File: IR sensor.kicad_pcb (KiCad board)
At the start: 2 copper layers, 33.5 x 16.8 mm, 23 parts, among them P1 BNC, P2 BNC, P3 BNC, P4 CONN_01X02, Q1 SOT-23-3 NPN, U1 TLV2770IDGKR, U2 LM311MX/NOPB

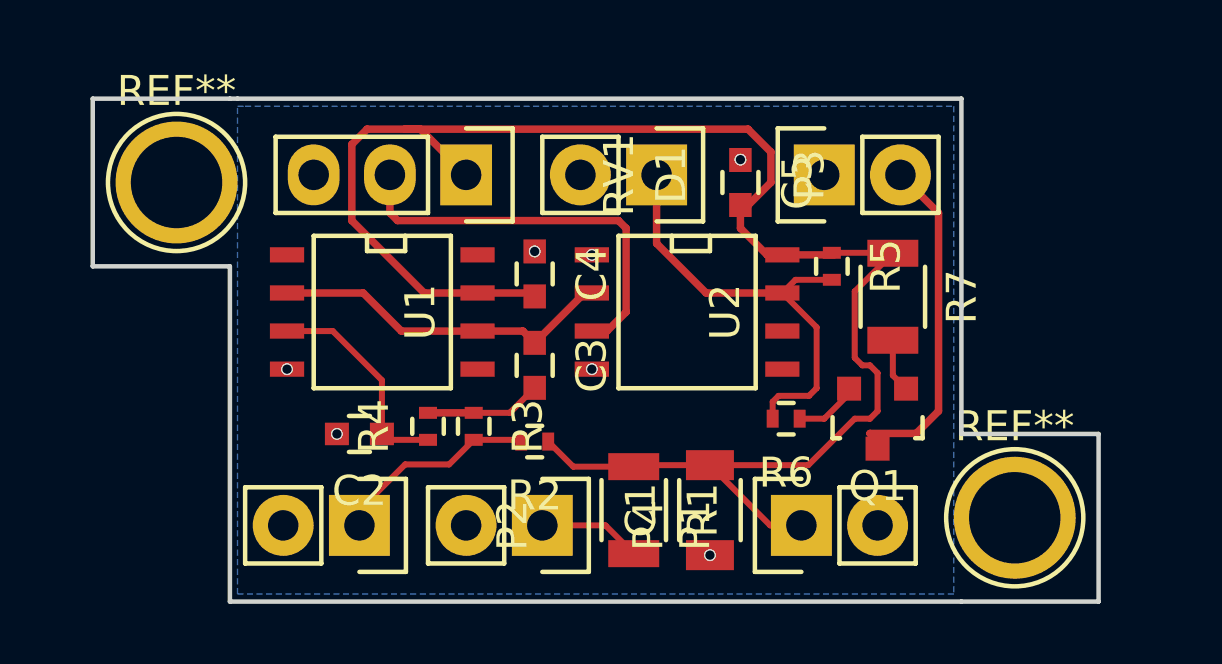
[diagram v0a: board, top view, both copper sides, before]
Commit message: ENH: Updates to IR sensors
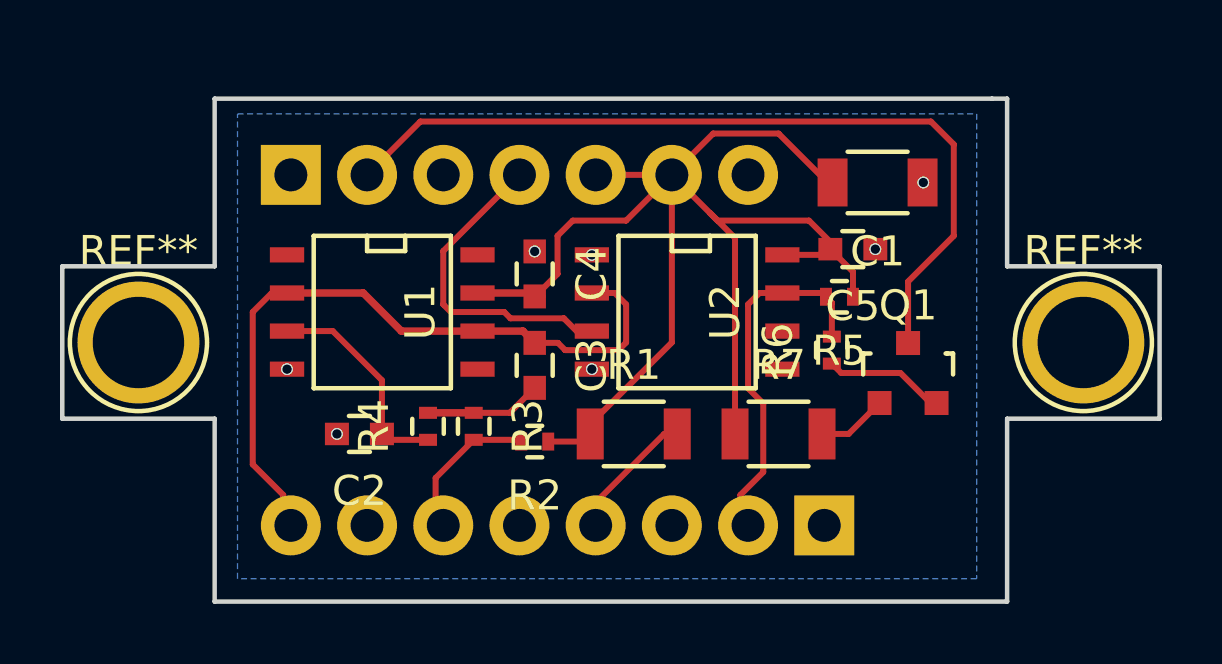
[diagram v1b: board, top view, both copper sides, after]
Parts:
- removed D1: LED, Pin_Headers:Pin_Header_Straight_1x02
- removed P3: BNC, Pin_Headers:Pin_Header_Straight_1x02
- removed P4: CONN_01X02, Pin_Headers:Pin_Header_Straight_1x02
- removed the REF** at (142.0, 67.3)
- removed the REF** at (169.9, 78.5)
- removed RV1: POT, Pin_Headers:Pin_Header_Straight_1x03
- added REF**: 1pin, Connect:1pin, F.Cu at (172.2, 72.6)
- added REF**: 1pin, Connect:1pin, F.Cu at (140.7, 72.6)
- P1: value BNC -> CONN_01X08; footprint Pin_Headers:Pin_Header_Straight_1x02 -> Terminal_Blocks:TerminalBlock_Pheonix_MPT-2.54mm_8pol; moved to B.Cu
- P2: value BNC -> CONN_01X07; footprint Pin_Headers:Pin_Header_Straight_1x02 -> Terminal_Blocks:TerminalBlock_Pheonix_MPT-2.54mm_7pol; moved to B.Cu
- U1: value TLV2770IDGKR -> TLV2770
- U2: value LM311MX/NOPB -> LM311
- moved C1 12.3 mm to (165.4, 67.3), turned to 180 degrees
- moved P2 11.9 mm to (145.8, 67.1), turned to 0 degrees
- moved P1 9.40 mm to (163.6, 78.7), turned to 180 degrees
- moved R7 5.95 mm to (162.1, 75.7), turned to 0 degrees
- moved C5 4.36 mm to (164.5, 69.5), turned to 180 degrees
- moved R6 2.75 mm to (163.8, 72.9), turned to 90 degrees
- moved R1 2.54 mm to (157.2, 75.7), turned to 0 degrees
- moved Q1 1.83 mm to (166.4, 73.7), turned to 0 degrees
- moved R5 1.05 mm to (164.1, 71.1), turned to 180 degrees
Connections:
- C3 pad 1: Net-(C3-Pad1) -> IR+
- P1 pad 1: Net-(P1-Pad1) -> GND
- P1 pad 2: GND -> TTL+
- P2 pad 1: Net-(P2-Pad1) -> GND
- P2 pad 2: GND -> LED+
- Q1 pad 3: Net-(D1-Pad2) -> LED+
- R1 pad 2: Net-(P1-Pad1) -> E+
- R2 pad 2: Net-(P2-Pad1) -> S+
- R3 pad 2: Net-(P2-Pad1) -> S+
- R5 pad 2: Net-(P3-Pad1) -> TTL+
- R6 pad 2: Net-(P3-Pad1) -> TTL+
- U1 pad 2: Net-(C3-Pad1) -> IR+
- U1 pad 6: Net-(C3-Pad1) -> IR+
- U2 pad 2: Net-(C3-Pad1) -> IR+
- U2 pad 3: Net-(RV1-Pad2) -> POT2
- U2 pad 7: Net-(P3-Pad1) -> TTL+
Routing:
- net LED+: track 0.00 -> 27.9 mm
- net IR+: track 0.00 -> 23.4 mm
- net Net-(P3-Pad1): track 15.4 -> 0.00 mm
- net Net-(RV1-Pad2): track 13.6 -> 0.00 mm
- net TTL+: track 0.00 -> 12.1 mm
- net Net-(C3-Pad1): track 11.5 -> 0.00 mm
- net Net-(D1-Pad2): track 11.4 -> 0.00 mm
- net POT2: track 0.00 -> 10.7 mm
- net +5V: track 57.9 -> 49.6 mm
- net Net-(P2-Pad1): track 6.95 -> 0.00 mm
- net S+: track 0.00 -> 4.53 mm
- net E+: track 0.00 -> 4.03 mm
- net Net-(P1-Pad1): track 3.44 -> 0.00 mm
- net Net-(Q1-Pad2): track 2.16 -> 4.03 mm
- net Net-(Q1-Pad1): track 1.80 -> 2.35 mm
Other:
- board size 33.5 x 16.8 mm -> 36.6 x 16.8 mm
- board text added: "5V"
- board text added: "LED"
- board text added: "P1"
- board text added: "P2"
- board text added: "P3"
- board text removed: "POT"
- board text removed: "PWR"
